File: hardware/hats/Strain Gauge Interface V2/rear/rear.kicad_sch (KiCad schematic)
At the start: 75 parts, among them J1 Conn_01x14, U1 ADS1235IRHBT, U2 ADS1235IRHBT, U3 LMR50410YQDBVRQ1, U5 BD450, U6 BD433

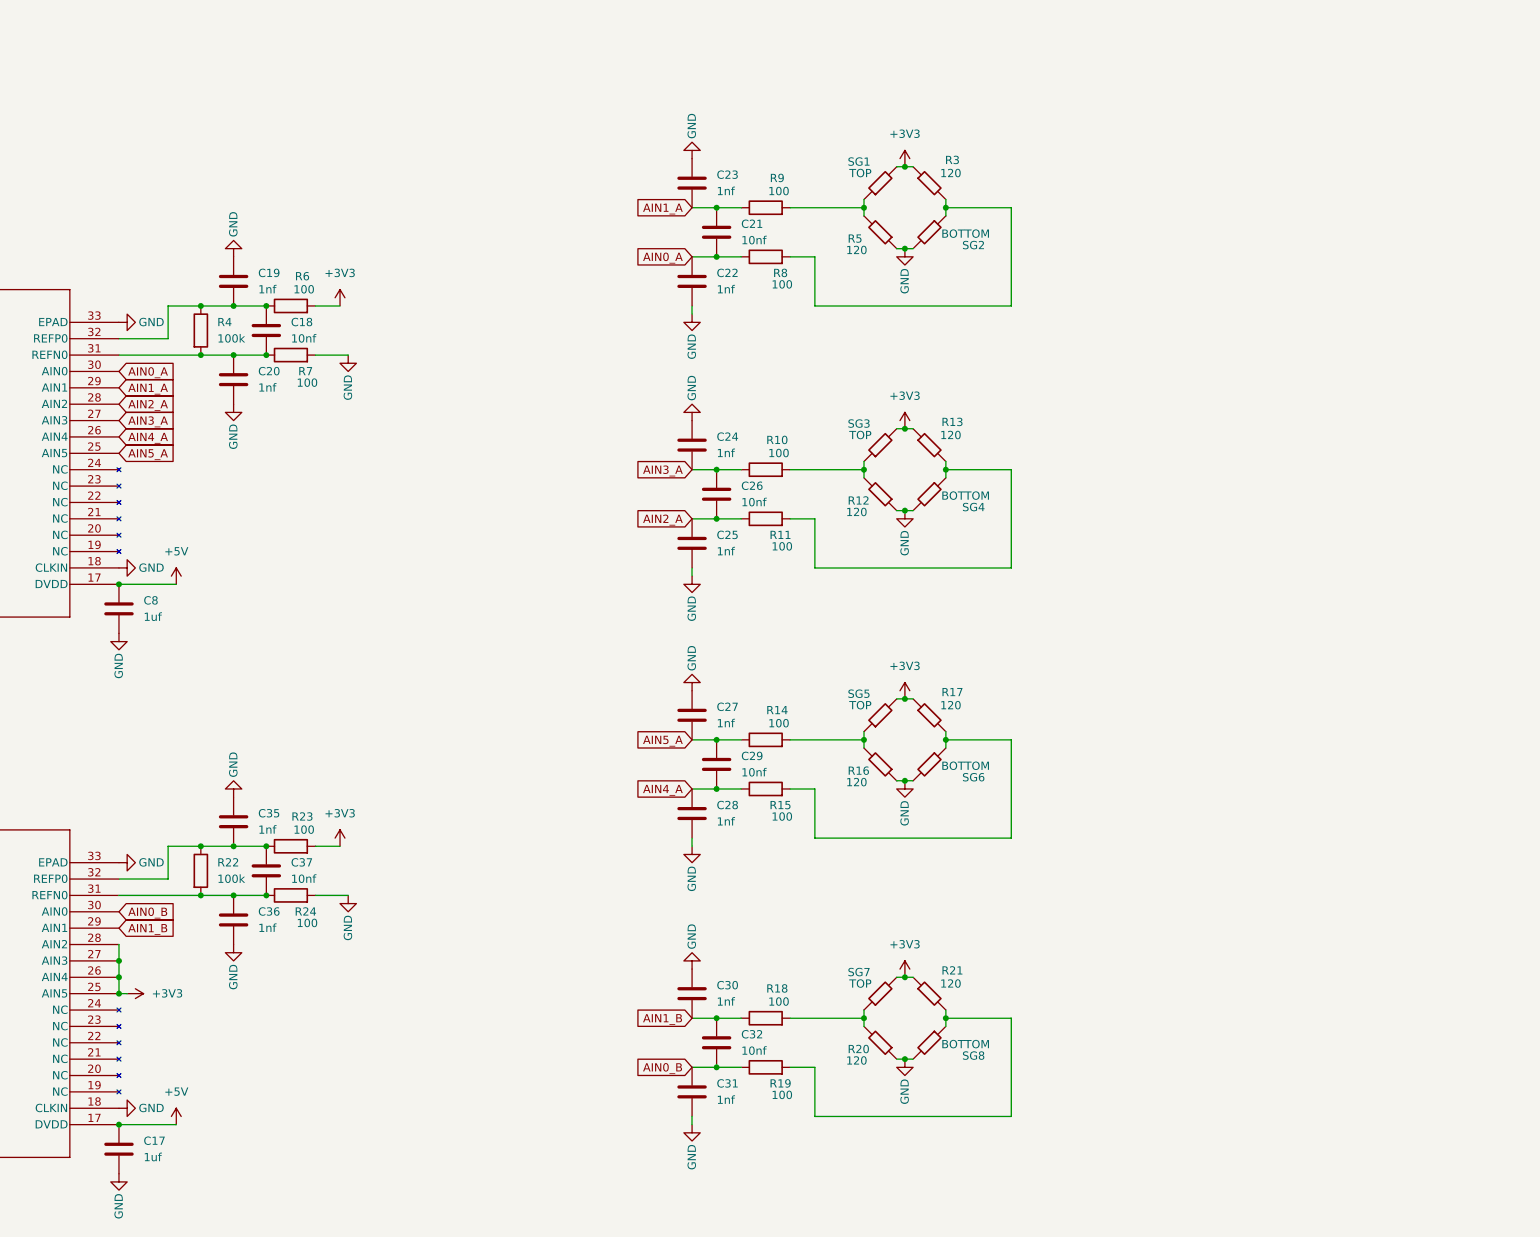
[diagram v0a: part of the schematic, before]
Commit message: 6 wishbones
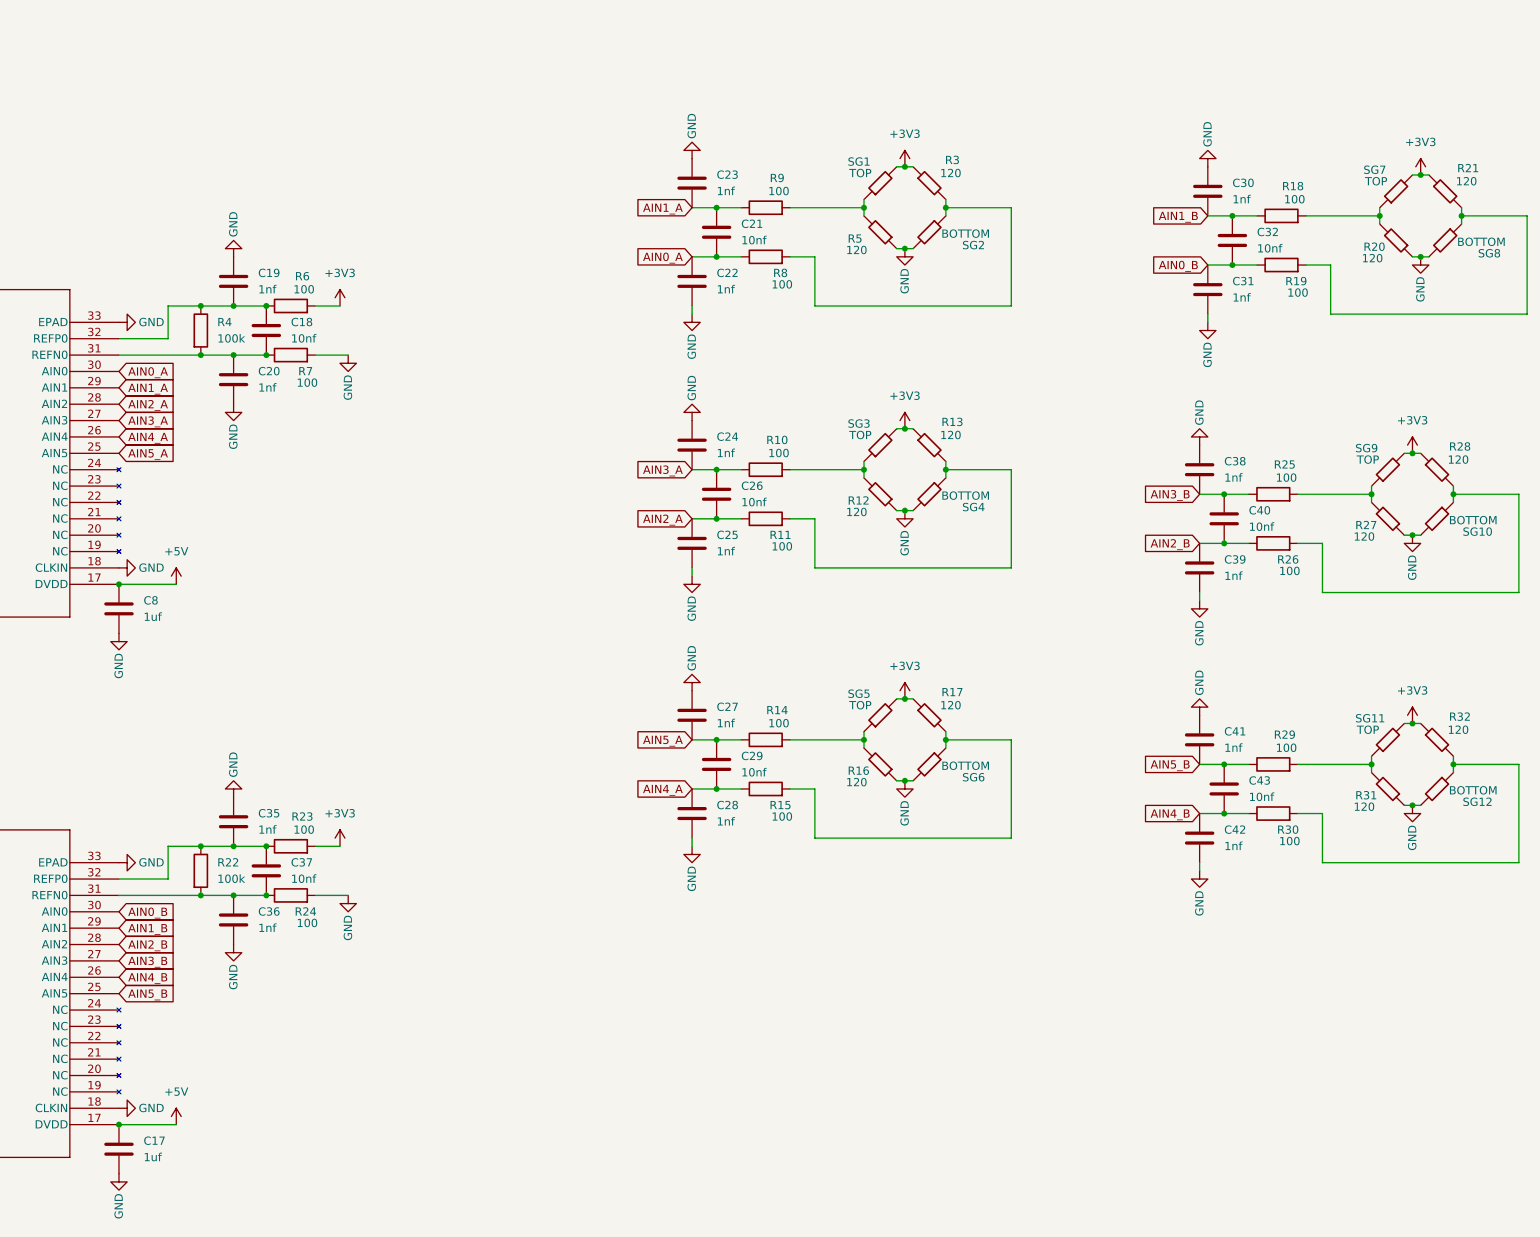
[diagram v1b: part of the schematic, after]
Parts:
- added C38, C39, C41, C42: 1nf, Capacitor_SMD:C_0603_1608Metric, symbol Device:C
- added C40, C43: 10nf, Capacitor_SMD:C_0603_1608Metric, symbol Device:C
- added R25, R26, R29, R30: 100, Resistor_SMD:R_0603_1608Metric, symbol Device:R
- added R27, R28, R31, R32: 120, Resistor_SMD:R_0603_1608Metric, symbol Device:R_45deg
- added SG10, SG12: BOTTOM, Connector_JST:JST_XA_S02B-XASK-1_1x02_P2.50mm_Horizontal, symbol Device:R_45deg
- added SG11, SG9: TOP, Connector_JST:JST_XA_S02B-XASK-1_1x02_P2.50mm_Horizontal, symbol Device:R_45deg
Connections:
- net +3V3: now also R28.1, R32.1, SG11.2, SG9.2; no longer U2.25 (AIN5), U2.26 (AIN4), U2.27 (AIN3), U2.28 (AIN2)
- net GND: now also C38.1, C39.2, C41.1, C42.2, R27.1, R31.1, SG10.2, SG12.2
- new net: R26.2, R28.2, SG10.1
- new net: R25.2, R27.2, SG9.1
- new net: R30.2, R32.2, SG12.1
- new net: R29.2, R31.2, SG11.1
- new net AIN2_B: C39.1, C40.2, R26.1, U2.28 (AIN2)
- new net AIN3_B: C38.2, C40.1, R25.1, U2.27 (AIN3)
- new net AIN4_B: C42.1, C43.2, R30.1, U2.26 (AIN4)
- new net AIN5_B: C41.2, C43.1, R29.1, U2.25 (AIN5)
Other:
- moved on the sheet: C30, C31, C32, R18, R19, R20, R21, SG7, SG8

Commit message: this is worse than torture
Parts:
- removed C10, C11, C12, C13, C14, C15, C17, C8: 1uf, Capacitor_SMD:C_0603_1608Metric, symbol Device:C
- removed C16, C18, C21, C26, C29, C32, C37, C40, C43, C9: 10nf, Capacitor_SMD:C_0603_1608Metric, symbol Device:C
- removed C19, C20, C22, C23, C24, C25, C27, C28, C30, C31, C35, C36, C38, C39, C41, C42: 1nf, Capacitor_SMD:C_0603_1608Metric, symbol Device:C
- removed R10, R11, R14, R15, R18, R19, R23, R24, R25, R26, R29, R30, R6, R7, R8, R9: 100, Resistor_SMD:R_0603_1608Metric, symbol Device:R
- removed R12, R13, R16, R17, R20, R21, R27, R28, R3, R31, R32, R5: 120, Resistor_SMD:R_0603_1608Metric, symbol Device:R_45deg
- removed R22, R4: 100k, Resistor_SMD:R_0603_1608Metric, symbol Device:R
- removed SG1, SG11, SG3, SG5, SG7, SG9: TOP, Connector_JST:JST_XA_S02B-XASK-1_1x02_P2.50mm_Horizontal, symbol Device:R_45deg
- removed SG10, SG12, SG2, SG4, SG6, SG8: BOTTOM, Connector_JST:JST_XA_S02B-XASK-1_1x02_P2.50mm_Horizontal, symbol Device:R_45deg
- removed U1, U2: ADS1235IRHBT, CustomFootprints:RHB32_TEX, symbol STRAINGAUGEADC:ADS1235IRHBT
- added C100, C104, C105, C106, C107, C108, C109, C118, C119, C126, C127, C54, C55, C56, C57, C65, C66, C68, C69, C70, C71, C72, C73, C77, C78, C79, C80, C81, C82, C86, C87, C88, C89, C90, C91, C95, C96, C97, C98, C99: 1nf, Capacitor_SMD:C_0603_1608Metric, symbol Device:C
- added C101, C102, C103, C110, C111, C112, C116, C120, C124, C128, C50, C51, C58, C59, C63, C67, C74, C75, C76, C83, C84, C85, C92, C93, C94: 10nf, Capacitor_SMD:C_0603_1608Metric, symbol Device:C
- added C113, C114, C115, C117, C121, C122, C123, C125, C44, C45, C46, C47, C48, C49, C52, C53, C60, C61, C62, C64: 1uf, Capacitor_SMD:C_0603_1608Metric, symbol Device:C
- added R100, R101, R102, R103, R104, R105, R106, R107, R108, R109, R110, R111, R112, R113, R114, R115, R116, R48, R49, R50, R51, R52, R53, R60, R61, R62, R63, R64, R65, R72, R73, R74, R75, R76, R77, R84, R85, R86, R87, R88, R89, R96, R97, R98, R99: 120, Resistor_SMD:R_0603_1608Metric, symbol Device:R_45deg
- added R117, R120, R33, R34, R39: 100k, Resistor_SMD:R_0603_1608Metric, symbol Device:R
- added R118, R119, R121, R122, R35, R36, R37, R38, R40, R41, R42, R43, R44, R45, R46, R47, R54, R55, R56, R57, R58, R59, R66, R67, R68, R69, R70, R71, R78, R79, R80, R81, R82, R83, R90, R91, R92, R93, R94, R95: 100, Resistor_SMD:R_0603_1608Metric, symbol Device:R
- added SG13, SG19, SG25, SG31, SG37: 45D, Connector_JST:JST_XA_S02B-XASK-1_1x02_P2.50mm_Horizontal, symbol Device:R_45deg
- added SG14, SG20, SG26, SG32, SG38: 90D, Connector_JST:JST_XA_S02B-XASK-1_1x02_P2.50mm_Horizontal, symbol Device:R_45deg
- added SG15, SG21, SG27, SG33, SG39: 0D, Connector_JST:JST_XA_S02B-XASK-1_1x02_P2.50mm_Horizontal, symbol Device:R_45deg
- added U10, U4, U7, U8, U9: ADS1235IRHBT, CustomFootprints:RHB32_TEX, symbol STRAINGAUGEADC:ADS1235IRHBT
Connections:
- net +3V3: now also R100.1, R101.1, R118.2, R121.2, R35.2, R37.2, R40.2, R51.1, R52.1, R53.1, R63.1, R64.1, R65.1, R75.1, R76.1, R77.1, R87.1, R88.1, R89.1, R99.1, SG13.2, SG14.2, SG15.2, SG19.2, SG20.2, SG21.2, SG25.2, SG26.2, SG27.2, SG31.2, SG32.2, SG33.2, SG37.2, SG38.2, SG39.2
- net +5V: now also C117.1, C125.1, C52.1, C53.1, C64.1, U10.17 (DVDD), U10.7 (*PWDN), U10.8 (*RESET), U10.9 (START), U4.17 (DVDD), U4.7 (*PWDN), U4.8 (*RESET), U4.9 (START), U7.17 (DVDD), U7.7 (*PWDN), U7.8 (*RESET), U7.9 (START), U8.17 (DVDD), U8.7 (*PWDN), U8.8 (*RESET), U8.9 (START), U9.17 (DVDD), U9.7 (*PWDN), U9.8 (*RESET), U9.9 (START)
- net CS1: now also U4.10 (*CS)
- net CS2: now also U10.10 (*CS), U7.10 (*CS), U8.10 (*CS), U9.10 (*CS)
- net DIN: now also U10.12 (DIN), U4.12 (DIN), U7.12 (DIN), U8.12 (DIN), U9.12 (DIN)
- net DOUT: now also U10.14 (DOUT/*DRDY), U4.14 (DOUT/*DRDY), U7.14 (DOUT/*DRDY), U8.14 (DOUT/*DRDY), U9.14 (DOUT/*DRDY)
- net GND: now also C100.2, C104.1, C105.2, C106.1, C107.2, C108.1, C109.2, C113.2, C114.2, C115.2, C117.2, C118.1, C119.2, C121.2, C122.2, C123.2, C125.2, C126.1, C127.2, C44.2, C45.2, C46.2, C47.2, C48.2, C49.2, C52.2, C53.2, C54.1, C55.2, C56.1, C57.2, C60.2, C61.2, C62.2, C64.2, C65.1, C66.2, C68.1, C69.2, C70.1, C71.2, C72.1, C73.2, C77.1, C78.2, C79.1, C80.2, C81.1, C82.2, C86.1, C87.2, C88.1, C89.2, C90.1, C91.2, C95.1, C96.2, C97.1, C98.2, C99.1, R102.1, R103.2, R104.2, R105.2, R106.2, R107.1, R108.2, R109.2, R110.2, R111.2, R112.2, R113.2, R114.2, R115.2, R116.2, R119.2, R122.2, R36.2, R38.2, R41.2, R48.1, R49.1, R50.1, R60.1, R61.1, R62.1, R72.1, R73.1, R74.1, R84.1, R85.1, R86.1, R96.1, R97.1, R98.1, U10.16 (DGND), U10.18 (CLKIN), U10.33 (EPAD), U10.5 (AVSS), U4.16 (DGND), U4.18 (CLKIN), U4.33 (EPAD), U4.5 (AVSS), U7.16 (DGND), U7.18 (CLKIN), U7.33 (EPAD), U7.5 (AVSS), U8.16 (DGND), U8.18 (CLKIN), U8.33 (EPAD), U8.5 (AVSS), U9.16 (DGND), U9.18 (CLKIN), U9.33 (EPAD), U9.5 (AVSS)
- net SCLK: now also U10.11 (SCLK), U4.11 (SCLK), U7.11 (SCLK), U8.11 (SCLK), U9.11 (SCLK)
- new net: R100.2, R116.1, R93.2
- new net: R101.2, R114.1, R95.2
- new net: R107.2, R45.2, R52.2
- new net: R66.2, R72.2, SG25.1
- new net: C60.1, C61.1, U8.4 (AVDD)
- new net: C55.1, C58.2, R33.2, R36.1, U4.31 (REFN0)
- new net: R68.2, R73.2, SG26.1
- new net: C57.1, C59.2, R34.2, R38.1, U7.31 (REFN0)
- new net: C54.2, C58.1, R33.1, R35.1, U4.32 (REFP0)
- new net: C56.2, C59.1, R34.1, R37.1, U7.32 (REFP0)
- new net: C124.1, U10.2 (CAPP)
- new net: C124.2, U10.3 (CAPN)
- new net: R90.2, R96.2, SG37.1
- new net: C50.1, U4.2 (CAPP)
- new net: C50.2, U4.3 (CAPN)
- new net: R103.1, R59.2, R65.2
- new net: R70.2, R74.2, SG27.1
- new net: C126.2, C128.1, R120.1, R121.1, U10.32 (REFP0)
- new net: R44.2, R49.2, SG14.1
- new net: R46.2, R50.2, SG15.1
- new net: R115.1, R91.2, R99.2
- new net: C48.1, U4.15 (BYPASS)
- new net: R104.1, R55.2, R63.2
- new net: R110.1, R67.2, R75.2
- new net: C65.2, C67.1, R39.1, R40.1, U8.32 (REFP0)
- new net: C66.1, C67.2, R39.2, R41.1, U8.31 (REFN0)
- new net: R58.2, R62.2, SG21.1
- new net: C116.1, U9.2 (CAPP)
- new net: C116.2, U9.3 (CAPN)
- new net: R102.2, R47.2, R53.2
- new net: C62.1, U8.15 (BYPASS)
- new net: C118.2, C120.1, R117.1, R118.1, U9.32 (REFP0)
- new net: C119.1, C120.2, R117.2, R119.1, U9.31 (REFN0)
- new net: R54.2, R60.2, SG19.1
- new net: R105.1, R57.2, R64.2
- new net: R111.1, R79.2, R87.2
- new net: R56.2, R61.2, SG20.1
- new net: C127.1, C128.2, R120.2, R122.1, U10.31 (REFN0)
- new net: R82.2, R86.2, SG33.1
- new net: C44.1, C46.1, U4.4 (AVDD)
- new net: R109.1, R83.2, R89.2
- new net: R113.1, R81.2, R88.2
- new net: C113.1, C114.1, U9.4 (AVDD)
- new net: C49.1, U7.15 (BYPASS)
- new net: C51.1, U7.2 (CAPP)
- new net: C51.2, U7.3 (CAPN)
- new net: C45.1, C47.1, U7.4 (AVDD)
- new net: C115.1, U9.15 (BYPASS)
- new net: R78.2, R84.2, SG31.1
- new net: C121.1, C122.1, U10.4 (AVDD)
- new net: R92.2, R97.2, SG38.1
- new net: R94.2, R98.2, SG39.1
- new net: R108.1, R71.2, R77.2
- new net: R42.2, R48.2, SG13.1
- new net: R80.2, R85.2, SG32.1
- new net: C63.1, U8.2 (CAPP)
- new net: C63.2, U8.3 (CAPN)
- new net: R106.1, R43.2, R51.2
- new net: C123.1, U10.15 (BYPASS)
- new net: R112.1, R69.2, R76.2
- new net AIN0_C: C73.1, C76.2, R47.1, U4.30 (AIN0)
- new net AIN0_D: C82.1, C85.2, R59.1, U7.30 (AIN0)
- new net AIN0_E: C91.1, C94.2, R71.1, U8.30 (AIN0)
- new net AIN0_F: C100.1, C103.2, R83.1, U9.30 (AIN0)
- new net AIN0_G: C109.1, C112.2, R95.1, U10.30 (AIN0)
- new net AIN1_C: C72.2, C76.1, R46.1, U4.29 (AIN1)
- new net AIN1_D: C81.2, C85.1, R58.1, U7.29 (AIN1)
- new net AIN1_E: C90.2, C94.1, R70.1, U8.29 (AIN1)
- new net AIN1_F: C103.1, C99.2, R82.1, U9.29 (AIN1)
- new net AIN1_G: C108.2, C112.1, R94.1, U10.29 (AIN1)
- new net AIN2_C: C69.1, C74.2, R43.1, U4.28 (AIN2)
- new net AIN2_D: C78.1, C83.2, R55.1, U7.28 (AIN2)
- new net AIN2_E: C87.1, C92.2, R67.1, U8.28 (AIN2)
- new net AIN2_F: C101.2, C96.1, R79.1, U9.28 (AIN2)
- new net AIN2_G: C105.1, C110.2, R91.1, U10.28 (AIN2)
- new net AIN3_C: C68.2, C74.1, R42.1, U4.27 (AIN3)
- new net AIN3_D: C77.2, C83.1, R54.1, U7.27 (AIN3)
- new net AIN3_E: C86.2, C92.1, R66.1, U8.27 (AIN3)
- new net AIN3_F: C101.1, C95.2, R78.1, U9.27 (AIN3)
- new net AIN3_G: C104.2, C110.1, R90.1, U10.27 (AIN3)
- new net AIN4_C: C71.1, C75.2, R45.1, U4.26 (AIN4)
- new net AIN4_D: C80.1, C84.2, R57.1, U7.26 (AIN4)
- new net AIN4_E: C89.1, C93.2, R69.1, U8.26 (AIN4)
- new net AIN4_F: C102.2, C98.1, R81.1, U9.26 (AIN4)
- new net AIN4_G: C107.1, C111.2, R93.1, U10.26 (AIN4)
- new net AIN5_C: C70.2, C75.1, R44.1, U4.25 (AIN5)
- new net AIN5_D: C79.2, C84.1, R56.1, U7.25 (AIN5)
- new net AIN5_E: C88.2, C93.1, R68.1, U8.25 (AIN5)
- new net AIN5_F: C102.1, C97.2, R80.1, U9.25 (AIN5)
- new net AIN5_G: C106.2, C111.1, R92.1, U10.25 (AIN5)
- no-connect marks 9 -> 12
